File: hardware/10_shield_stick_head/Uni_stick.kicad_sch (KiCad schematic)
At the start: 54 parts, among them IC1 MPX5050DP, IC2 MPX5050DP, J1 Conn_01x04, J2 Conn_01x04, J3 Conn_01x06, J4 Micro match 6x2, J5 Conn_01x04, J6 Conn_01x06, J7 Conn_01x04, J8 Conn_01x06, U1 MPXH6115A, U2 MPXH6115A

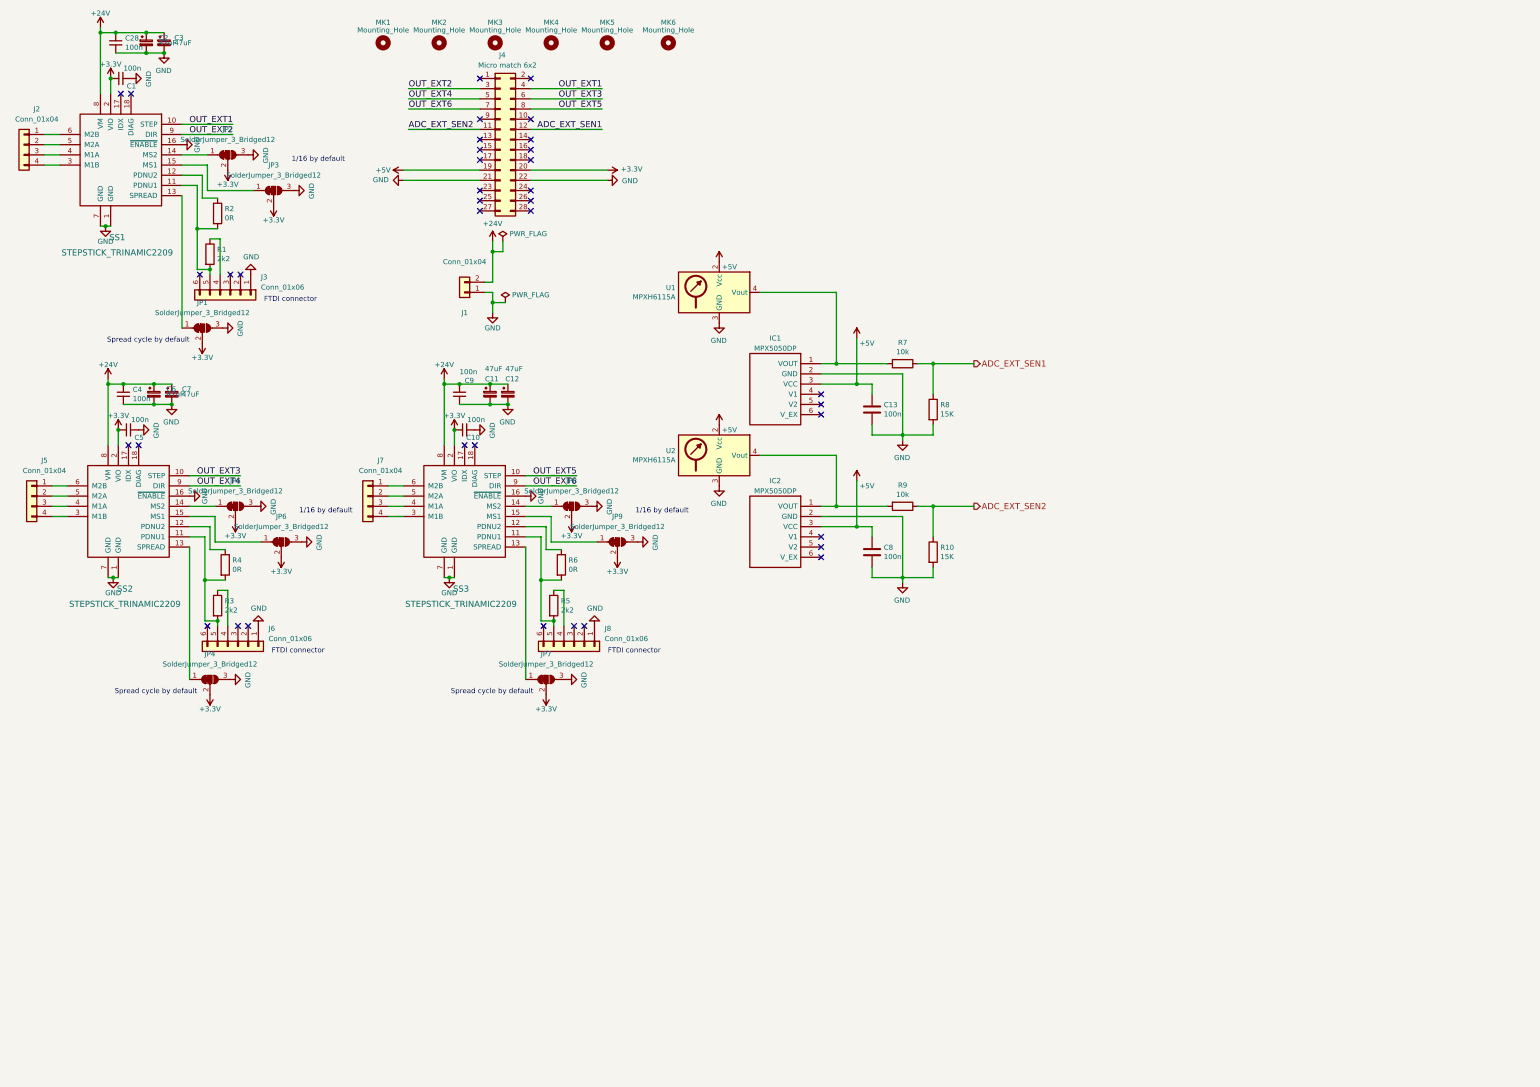
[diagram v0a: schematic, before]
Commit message: FW and SW updates for new revision
Signed-off-by: Jarosław Karwik <jaroslaw.karwik@gmail.com>
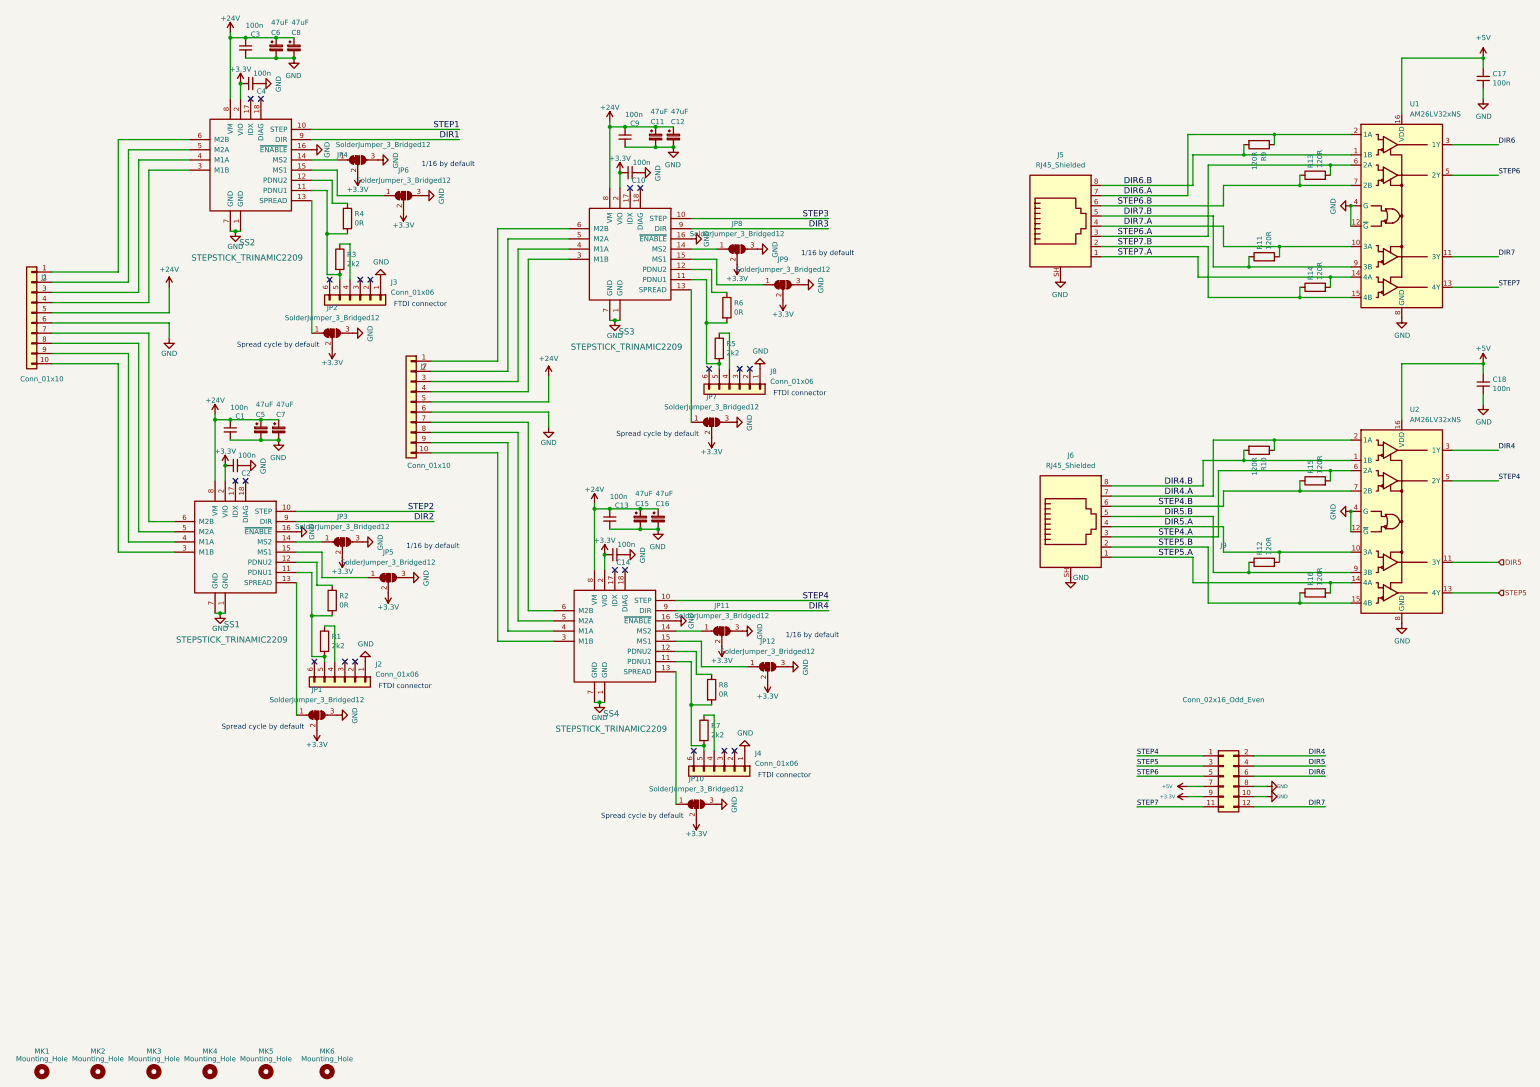
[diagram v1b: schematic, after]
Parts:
- removed C13, C8: 100n, Capacitor_SMD:C_0603_1608Metric, symbol Uni_stick-rescue:C-Device-Uni_stick-rescue
- removed C2, C3: 47uF, Capacitor_Tantalum_SMD:CP_EIA-7343-43_Kemet-X, symbol Uni_stick-rescue:CP_Small-Device-Uni_stick-rescue
- removed C28, C5: 100n, Capacitor_SMD:C_0603_1608Metric, symbol Uni_stick-rescue:C_Small-Device-Uni_stick-rescue
- removed IC1, IC2: MPX5050DP, Biblioteki:Pressure_sensor_v2, symbol Uni_stick-rescue:MPX5010DP-MPX5010DP
- removed J1: Conn_01x04, Connector_Phoenix_MC:PhoenixContact_MCV_1,5_2-G-3.5_1x02_P3.50mm_Vertical, symbol Connector_Generic:Conn_01x02
- removed J2, J5: Conn_01x04, Connector_Phoenix_MC:PhoenixContact_MCV_1,5_4-G-3.5_1x04_P3.50mm_Vertical, symbol Uni_stick-rescue:Conn_01x04-Connector_Generic-Uni_stick-rescue
- removed J4: Micro match 6x2, Connector_PinHeader_2.54mm:PinHeader_2x14_P2.54mm_Vertical, symbol Connector_Generic:Conn_02x14_Odd_Even
- removed J6: Conn_01x06, Connector_PinHeader_2.54mm:PinHeader_1x06_P2.54mm_Vertical, symbol Uni_stick-rescue:Conn_01x06-Connector_Generic-Uni_stick-rescue
- removed R10: 15K, Resistor_SMD:R_0603_1608Metric, symbol Uni_stick-rescue:R-Device-Uni_stick-rescue
- removed R9: 10k, Resistor_SMD:R_0603_1608Metric, symbol Uni_stick-rescue:R-Device-Uni_stick-rescue
- removed U1, U2: MPXH6115A, Biblioteki:MPXH6115AC6U, symbol Sensor_Pressure:MPXH6115A
- added C13, C14, C2, C3: 100n, Capacitor_SMD:C_0603_1608Metric, symbol Uni_stick-rescue:C_Small-Device-Uni_stick-rescue
- added C15, C5: 47uF, Capacitor_Tantalum_SMD:CP_EIA-7343-43_Kemet-X, symbol Uni_stick-rescue:CP_Small-Device-Uni_stick-rescue
- added C16, C8: 47uF, Capacitor_THT:CP_Radial_D8.0mm_P2.50mm, symbol Uni_stick-rescue:CP_Small-Device-Uni_stick-rescue
- added C17, C18: 100n, Capacitor_SMD:C_0603_1608Metric, symbol Uni_Printer-rescue:C_Small-Device
- added J1: Conn_01x10, Biblioteki:PhoenixContact_MC-G_10x3.50mm_Angled, symbol Connector_Generic:Conn_01x10
- added J2, J4: Conn_01x06, Connector_PinHeader_2.54mm:PinHeader_1x06_P2.54mm_Vertical, symbol Uni_stick-rescue:Conn_01x06-Connector_Generic-Uni_stick-rescue
- added J5, J6: RJ45_Shielded, Connector_RJ:RJ45_Ninigi_GE, symbol Connector:RJ45_Shielded
- added J9: Conn_02x16_Odd_Even, Connector_PinHeader_2.54mm:PinHeader_2x06_P2.54mm_Vertical, symbol Connector_Generic:Conn_02x06_Odd_Even
- added JP10, JP11, JP12: SolderJumper_3_Bridged12, Jumper:SolderJumper-3_P1.3mm_Bridged12_RoundedPad1.0x1.5mm, symbol Uni_stick-rescue:SolderJumper_3_Bridged12-Jumper-Uni_stick-rescue
- added R10, R11, R12, R13, R14, R15, R16, R9: 120R, Resistor_SMD:R_0603_1608Metric, symbol Uni_Printer-rescue:R-Device
- added SS4: STEPSTICK_TRINAMIC2209, Biblioteki:STEPSTICK, symbol Uni_stick-rescue:STEPSTICK_TRINAMIC2209-Uni_Printer-rescue-Uni_stick-rescue
- added U1, U2: AM26LV32xNS, Package_SO:SOIC-16W_5.3x10.2mm_P1.27mm, symbol Interface:AM26LV32xNS
- C12, C7: footprint Capacitor_Tantalum_SMD:CP_EIA-7343-43_Kemet-X -> Capacitor_THT:CP_Radial_D8.0mm_P2.50mm
- J7: value Conn_01x04 -> Conn_01x10; footprint Connector_Phoenix_MC:PhoenixContact_MCV_1,5_4-G-3.5_1x04_P3.50mm_Vertical -> Biblioteki:PhoenixContact_MC-G_10x3.50mm_Angled; symbol Uni_stick-rescue:Conn_01x04-Connector_Generic-Uni_stick-rescue -> Connector_Generic:Conn_01x10
- R7: value 10k -> 2k2; TME CRCW060310K0FKTABC -> WF06P-120R-5%
- R8: value 15K -> 0R; TME CQ0603-15K-1% -> WF06P-120R-5%
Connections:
- net +24V: now also C1.1, J7.5 (Pin_5), C13.1, C15.1, C16.1, C3.1, C5.1, C8.1, J1.5 (Pin_5), SS4.8 (VM); no longer C4.1
- net +3V3: now also C4.1, C14.1, C2.1, J9.9 (Pin_9), JP10.2 (C), JP11.2 (C), JP12.2 (C), SS4.2 (VIO); no longer C1.1
- net +5V: now also C17.1, C18.1, J9.7 (Pin_7), U1.16 (VDD), U2.16 (VDD)
- net GND: now also J7.6 (Pin_6), C13.2, C14.2, C15.2, C16.2, C17.2, C18.2, C2.2, C3.2, C5.2, C8.2, J1.6 (Pin_6), J2.1 (Pin_1), J4.1 (Pin_1), J5.SH, J6.SH, J9.10 (Pin_10), J9.8 (Pin_8), JP10.3 (B), JP11.3 (B), JP12.3 (B), SS4.1 (GND), SS4.16 (~{ENABLE}), SS4.7 (GND), U1.12 (~{G}), U1.4 (G), U1.8 (GND), U2.12 (~{G}), U2.4 (G), U2.8 (GND); no longer R8.2
- net at R1.2, R2.2, SS1.11 (PDNU1): now also J2.5 (Pin_5); no longer J3.5 (Pin_5)
- net at R1.1: now also J2.4 (Pin_4); no longer J3.4 (Pin_4)
- net at JP2.1 (A): now also SS2.13 (SPREAD); no longer SS1.14 (MS2)
- net at SS1.15 (MS1): now also JP5.1 (A); no longer JP3.1 (A)
- net at SS1.6 (M2B): now also J1.7 (Pin_7)
- net at SS1.5 (M2A): now also J1.8 (Pin_8)
- net at SS1.4 (M1A): now also J1.9 (Pin_9)
- net at SS1.3 (M1B): now also J1.10 (Pin_10)
- net at R3.1: now also J3.4 (Pin_4)
- net at R3.2, R4.2, SS2.11 (PDNU1): now also J3.5 (Pin_5)
- net at JP4.1 (A): now also SS2.14 (MS2); no longer SS2.13 (SPREAD)
- net at SS2.6 (M2B): now also J1.1 (Pin_1)
- net at SS2.5 (M2A): now also J1.2 (Pin_2)
- net at SS2.4 (M1A): now also J1.3 (Pin_3)
- net at SS2.3 (M1B): now also J1.4 (Pin_4)
- net at R7.2: now also R8.2, J4.5 (Pin_5), SS4.11 (PDNU1)
- net ADC_EXT_SEN1: no longer names the net of R8.1
- net ADC_EXT_SEN1: now also SS4.12 (PDNU2); no longer R7.1
- net OUT_EXT1 renamed STEP2
- net OUT_EXT2 renamed DIR2
- net OUT_EXT3 renamed STEP1
- net OUT_EXT4 renamed DIR1
- net OUT_EXT5 renamed STEP3
- net OUT_EXT6 renamed DIR3
- new net: J7.10 (Pin_10), SS4.3 (M1B)
- new net: J7.7 (Pin_7), SS4.6 (M2B)
- new net: J7.8 (Pin_8), SS4.5 (M2A)
- new net: J7.9 (Pin_9), SS4.4 (M1A)
- new net: JP10.1 (A), SS4.13 (SPREAD)
- new net: JP11.1 (A), SS4.14 (MS2)
- new net: JP12.1 (A), SS4.15 (MS1)
- new net: J4.4 (Pin_4), R7.1
- new net: JP3.1 (A), SS1.14 (MS2)
- new net DIR4: J9.2 (Pin_2), SS4.9 (DIR), U2.3 (1Y)
- new net DIR4.A: J6.7, R10.1, U2.2 (1A)
- new net DIR4.B: J6.8, R10.2, U2.1 (1B)
- new net DIR5: J9.4 (Pin_4), U2.11 (3Y)
- new net DIR5.A: J6.4, R12.2, U2.10 (3A)
- new net DIR5.B: J6.5, R12.1, U2.9 (3B)
- new net DIR6: J9.6 (Pin_6), U1.3 (1Y)
- new net DIR6.A: J5.7, R9.1, U1.2 (1A)
- new net DIR6.B: J5.8, R9.2, U1.1 (1B)
- new net DIR7: J9.12 (Pin_12), U1.11 (3Y)
- new net DIR7.A: J5.4, R11.2, U1.10 (3A)
- new net DIR7.B: J5.5, R11.1, U1.9 (3B)
- new net STEP4: J9.1 (Pin_1), SS4.10 (STEP), U2.5 (2Y)
- new net STEP4.A: J6.3, R15.2, U2.6 (2A)
- new net STEP4.B: J6.6, R15.1, U2.7 (2B)
- new net STEP5: J9.3 (Pin_3), U2.13 (4Y)
- new net STEP5.A: J6.1, R16.2, U2.14 (4A)
- new net STEP5.B: J6.2, R16.1, U2.15 (4B)
- new net STEP6: J9.5 (Pin_5), U1.5 (2Y)
- new net STEP6.A: J5.3, R13.2, U1.6 (2A)
- new net STEP6.B: J5.6, R13.1, U1.7 (2B)
- new net STEP7: J9.11 (Pin_11), U1.13 (4Y)
- new net STEP7.A: J5.1, R14.2, U1.14 (4A)
- new net STEP7.B: J5.2, R14.1, U1.15 (4B)
- no-connect marks 37 -> 20
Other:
- moved on the sheet: C10, C11, C12, C9, J8, JP7, JP8, JP9, MK1, MK2, MK3, MK4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
